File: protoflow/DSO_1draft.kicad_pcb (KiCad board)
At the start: 2 copper layers, 99.9 x 77.2 mm, 130 parts, among them J1 Conn_01x05, J2 Conn_Coaxial, J3 Conn_Coaxial, J4 Conn_Coaxial, J5 Conn_Coaxial, J7 USB_A_Stacked, J8 Conn_01x20, J9 Conn_01x20, SW1 SW_SPDT, SW2 SW_SPDT, SW3 SW_SPDT, SW4 SW_SPDT, SW5 SW_SPDT, U1 ADG708BRUZ, U2 ADG708BRUZ, U3 STM32G431C6Tx

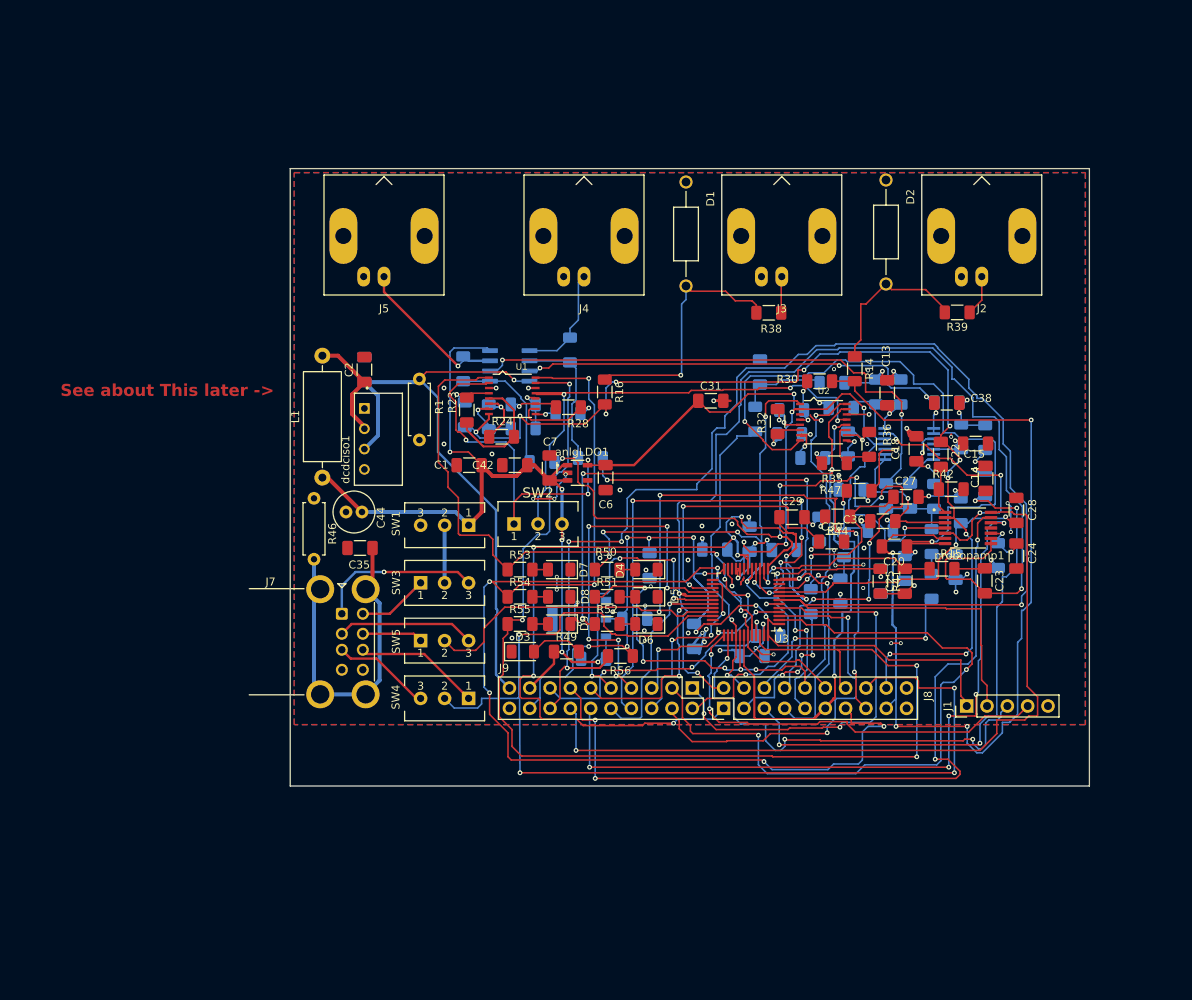
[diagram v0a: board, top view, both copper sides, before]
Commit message: final output
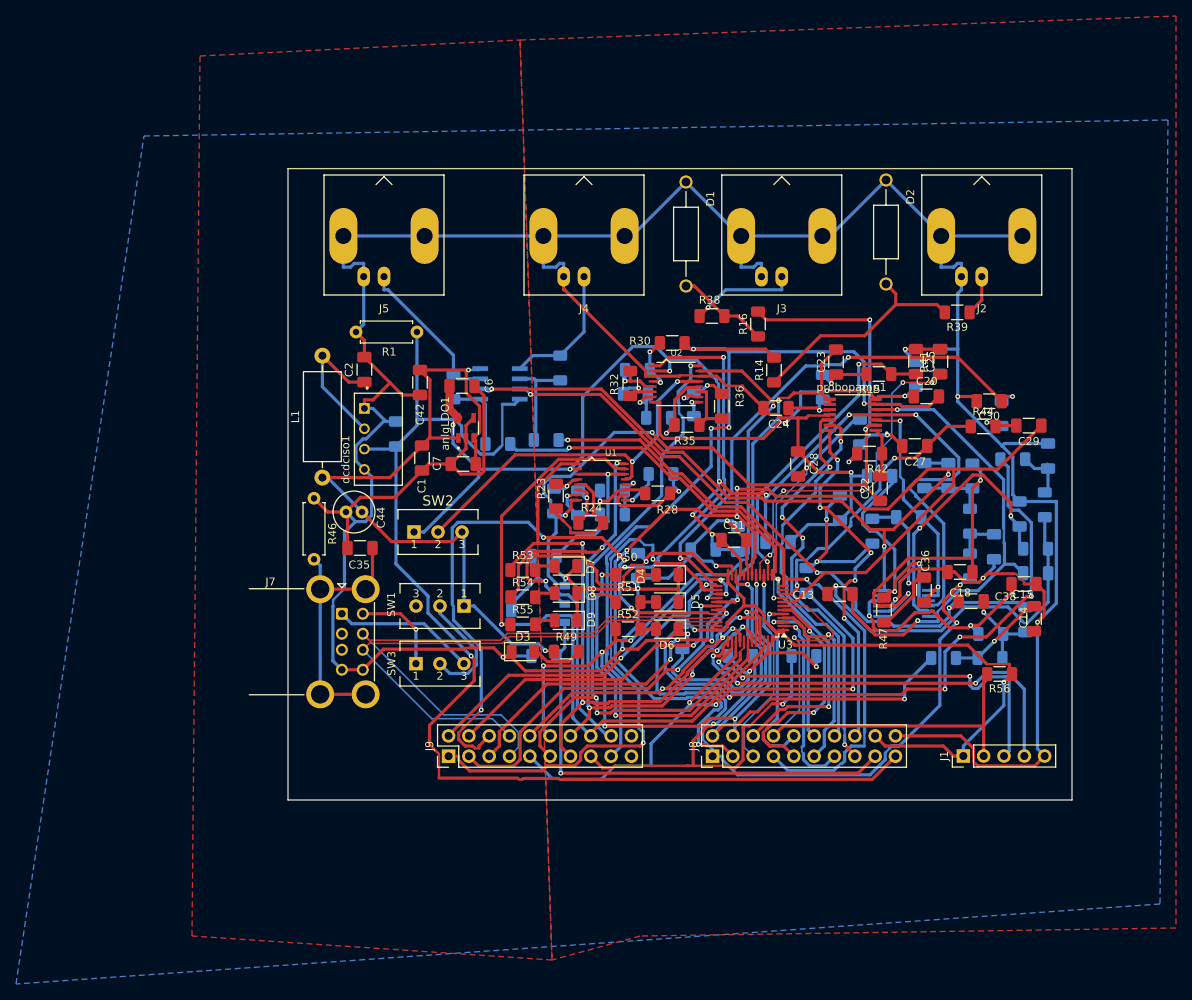
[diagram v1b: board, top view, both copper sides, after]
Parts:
- removed SW4, SW5: SW_SPDT, Slide_switch:SS-12F17_1P2T
- moved R56 47.5 mm to (171.9, 142.2)
- moved C11 37.5 mm to (178.0, 115.0)
- moved C24 35.3 mm to (144.0, 109.0), turned to 180 degrees
- moved J9 34.9 mm to (103.1, 152.5)
- moved C23 33.1 mm to (151.5, 103.2), turned to 90 degrees
- moved R5 32.6 mm to (173.6, 115.4), turned to 0 degrees
- moved C29 31.7 mm to (175.6, 111.2), turned to 0 degrees
- moved R6 30.7 mm to (177.6, 121.1), turned to -90 degrees
- moved R21 30.4 mm to (149.8, 106.4), turned to -90 degrees
- moved C16 28.9 mm to (175.2, 135.4), turned to 90 degrees
- moved R41 28.5 mm to (164.6, 103.2), turned to -90 degrees
- moved C26 28.4 mm to (164.5, 103.2), turned to 90 degrees
- moved C37 28.3 mm to (176.4, 129.7), turned to 180 degrees
- moved R7 28.0 mm to (176.4, 126.6), turned to 180 degrees
- moved C28 27.9 mm to (146.8, 116.0)
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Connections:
- J7 pad 2: Net-(J7-D1-) -> unconnected-(J7-D1--Pad2)
- J7 pad 3: Net-(J7-D1+) -> unconnected-(J7-D1+-Pad3)
- J7 pad 6: Net-(J7-D2-) -> /D-
- J7 pad 7: Net-(J7-D2+) -> /D+
- J8 pad 1: /PF0 -> /PB11_TM2_4
- J8 pad 10: /PA9 -> /PF0
- J8 pad 11: /PA10 -> /PC15
- J8 pad 12: /EOP+ -> /PC14
- J8 pad 13: /EOP- -> /PC13
- J8 pad 14: /EOP_OUT -> /EOP+
- J8 pad 15: /PB8 -> /EOP-
- J8 pad 16: /PG10_NRST -> /EOP_OUT
- J8 pad 2: /PF1 -> /PB10_TM2_3
- J8 pad 3: /PC13 -> /PA0_ADC_IN1
- J8 pad 4: /PC14 -> /B0
- J8 pad 5: /PC15 -> /PA7
- J8 pad 6: /PB12 -> /DAC2
- J8 pad 7: /PB14 -> /DAC1
- J8 pad 8: /PA7 -> /PG10_NRST
- J8 pad 9: /PA8 -> /PF1
- J9 pad 1: /PA0_ADC_IN1 -> /PB12
- J9 pad 10: /B1 -> /PB3_TM2_2
- J9 pad 11: /B2 -> /B1
- J9 pad 12: /A0 -> /B2
- J9 pad 13: /A1 -> /A0
- J9 pad 14: /A2 -> /A1
- J9 pad 15: /D- -> /PB8
- J9 pad 16: /D+ -> /A2
- J9 pad 2: /OP4_OUT -> /PB14
- J9 pad 3: /PB3_TM2_1 -> /OP4_OUT
- J9 pad 4: /PB3_TM2_2 -> /PA8
- J9 pad 5: /PB3_TM2_3 -> /PA9
- J9 pad 6: /PB3_TM2_4 -> /PA10
- J9 pad 7: /DAC1 -> /D-
- J9 pad 8: /DAC2 -> /D+
- J9 pad 9: /B0 -> /PA15_TM2_1
- R11 pad 1: /PB3_TM2_4 -> /PB11_TM2_4
- R4 pad 1: /PB3_TM2_1 -> /PA15_TM2_1
- R8 pad 1: /PB3_TM2_3 -> /PB10_TM2_3
- anlgLDO1 pad 4: unconnected-(anlgLDO1-NC-Pad4) -> GND
- digildo1 pad 4: (no net) -> /3v3_digi
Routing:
- net GND: track 76.3 -> 631.7 mm, vias 58 -> 15
- net /PG10_NRST: track 205.5 -> 64.4 mm, vias 4 -> 1
- net /A1: track 176.3 -> 83.1 mm, vias 8 -> 5
- net /PB11_TM2_4: track 0.00 -> 89.3 mm, vias 0 -> 3
- net /D+: track 142.7 -> 68.7 mm, vias 4 -> 0
- net /PA15_TM2_1: track 0.00 -> 72.8 mm, vias 0 -> 3
- net /-5v: track 75.5 -> 147.2 mm
- net /PB3_TM2_3: track 69.7 -> 0.00 mm, vias 4 -> 0
- net /PB3_TM2_2: track 38.3 -> 106.9 mm, vias 2 -> 7
- net /PC13: track 84.3 -> 23.4 mm, vias 2 -> 1
- net /B2: track 164.3 -> 103.7 mm, vias 4 -> 5
- net /A2: track 146.6 -> 86.0 mm, vias 4 -> 1
- net /PB10_TM2_3: track 0.00 -> 57.5 mm, vias 0 -> 2
- net /EOP_OUT: track 96.3 -> 45.2 mm, vias 1 -> 5
- net /OP4_OUT: track 140.1 -> 89.8 mm
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- added copper zone on F.Cu, net /3v3
- added copper zone on F.Cu, net /5v
- removed copper zone on F.Cu, net GND
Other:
- board size 99.9 x 77.2 mm -> 98 x 78.9 mm
- board text removed: "See about This later ->"
